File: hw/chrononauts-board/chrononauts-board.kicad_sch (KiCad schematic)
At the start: 56 parts, among them IC1 ESP32-C3-WROOM-02-N4, IC2 TLV62568DBVR, IC3 MXC6655XA, J1 73251-1290, J2 USB4105-GF-A, U1 CC1101RGP, Y1 NX3225GA-26MHZ

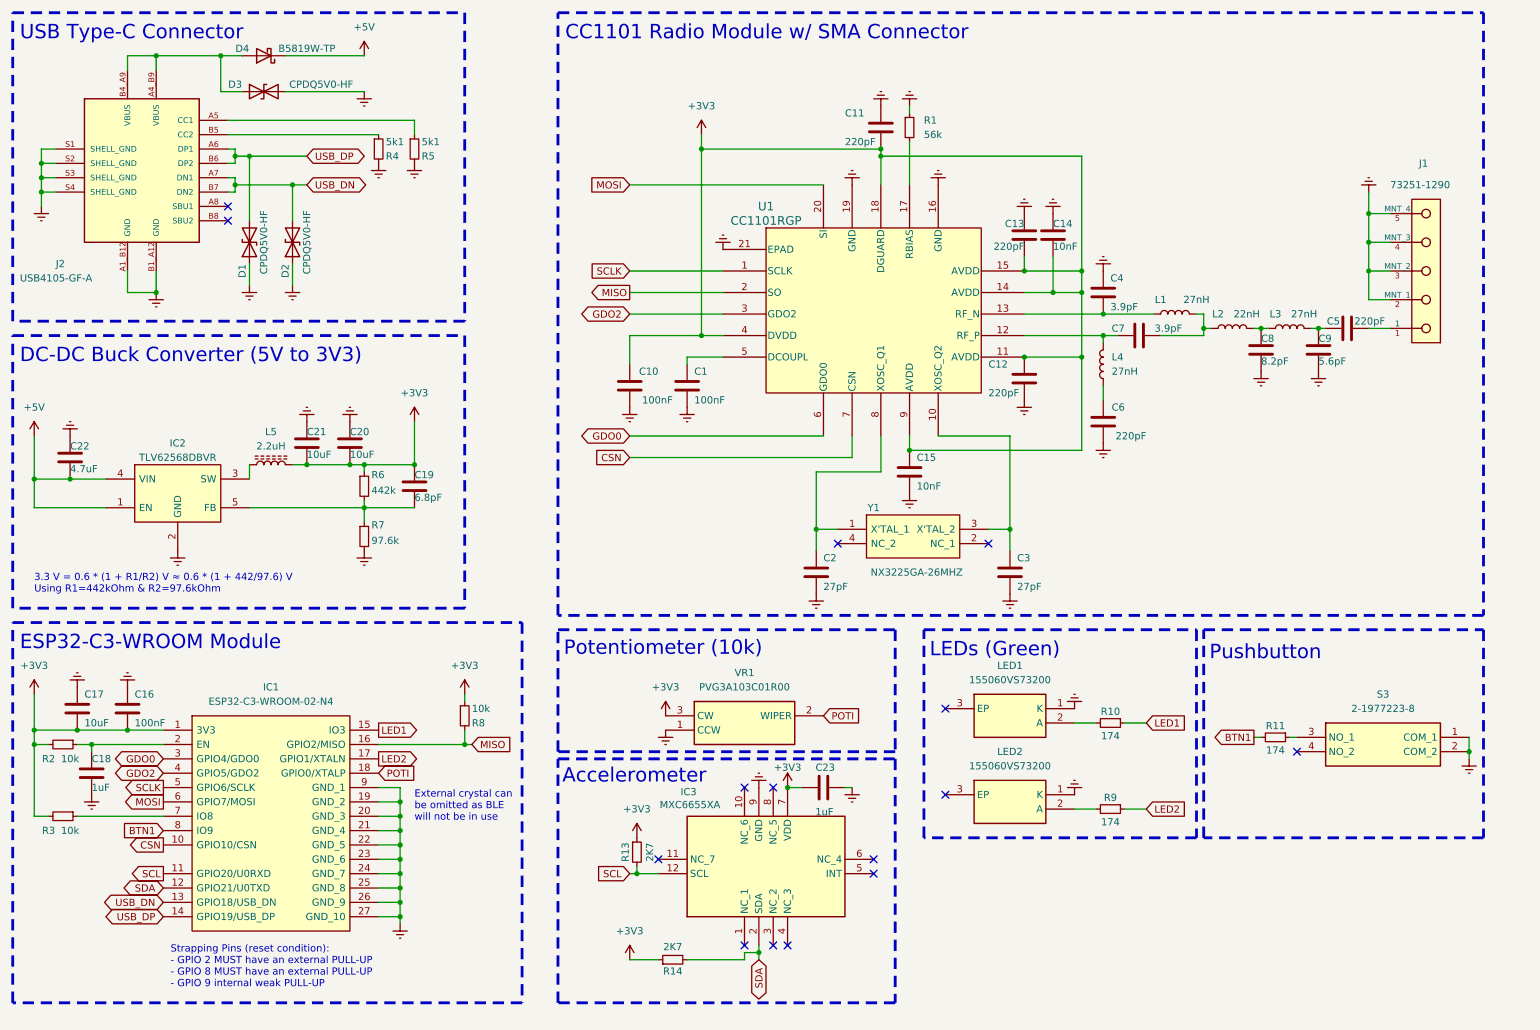
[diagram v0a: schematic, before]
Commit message: ready for production
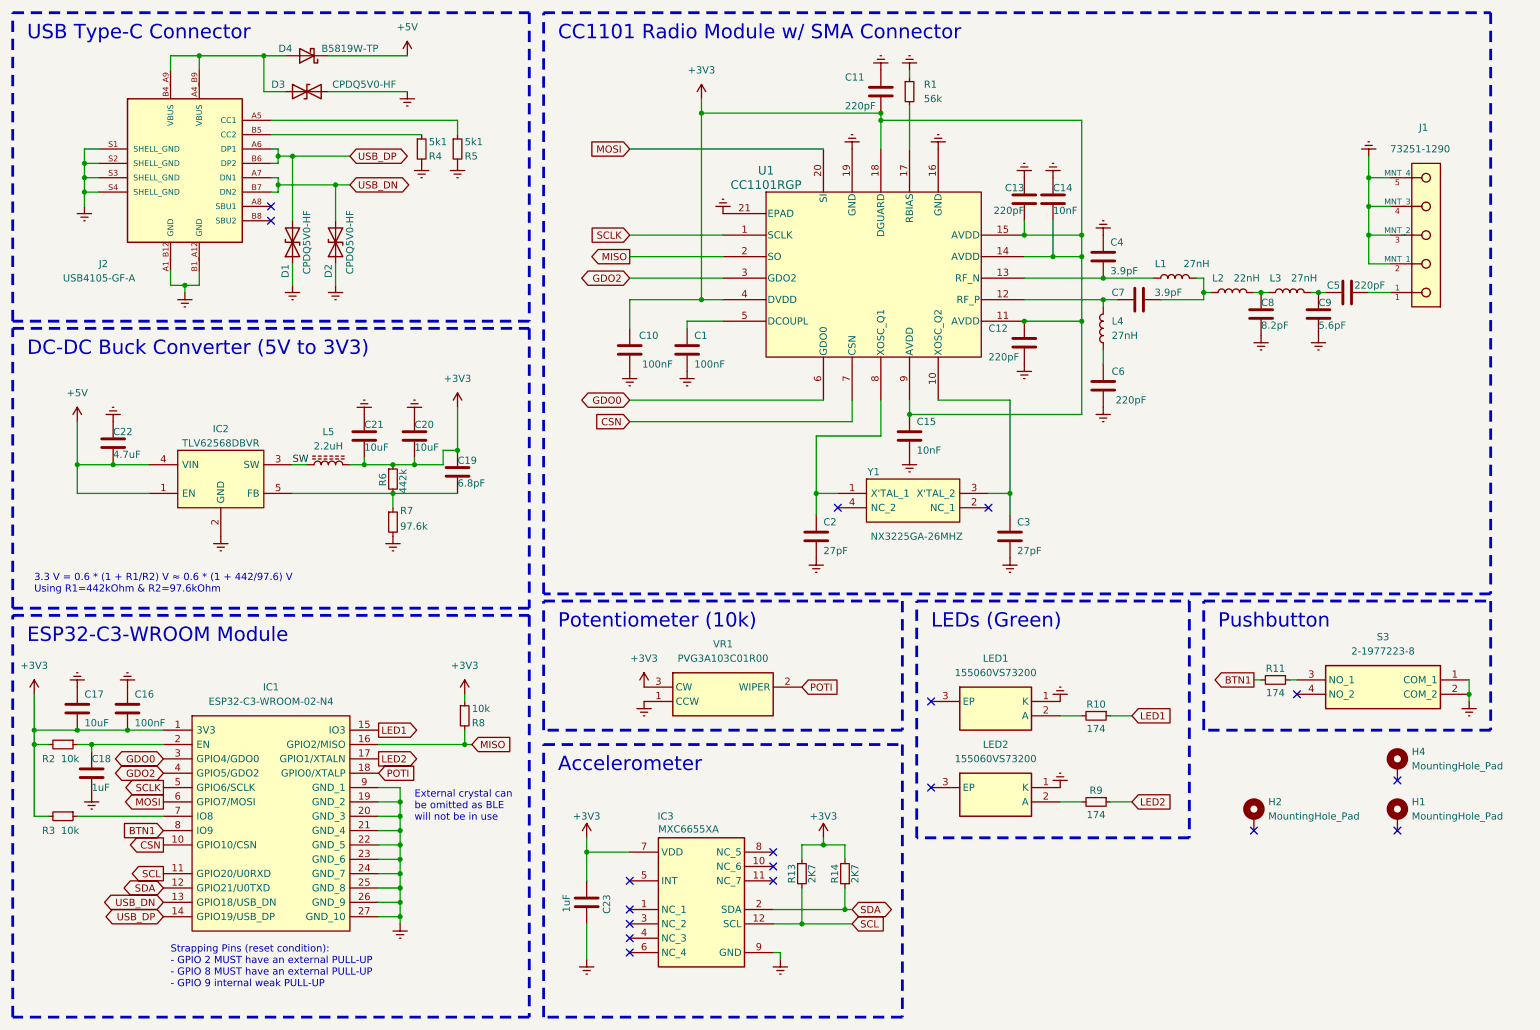
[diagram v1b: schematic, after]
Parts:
- added H1, H2, H4: MountingHole_Pad, MountingHole:MountingHole_2.2mm_M2_DIN965_Pad_TopBottom, symbol Mechanical:MountingHole_Pad
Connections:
- net +3V3: now also R14.2; no longer R14.1
- net SDA: now also R14.1; no longer R14.2
- net SW: now reaches IC2.3 (SW), L5.1
- no-connect marks 15 -> 18
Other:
- company: mineiwik -> chrononauts-quest
- moved on the sheet: C1, C10, C11, C12, C13, C14, C15, C19, C2, C20, C21, C22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

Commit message: generate production files
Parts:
- C1, C10, C16: LCSC (none) -> C431646
- C11, C12, C13, C5, C6: LCSC (none) -> C412611
- C14, C15: LCSC (none) -> C482489
- C17, C20, C21: LCSC (none) -> C510630
- C18, C23: LCSC (none) -> C527012
- C19: LCSC (none) -> C338054
- C2, C3: LCSC (none) -> C342944
- C22: LCSC (none) -> C77045
- C4, C7: LCSC (none) -> C565491
- C8: LCSC (none) -> C393674
- C9: LCSC (none) -> C525219
- D1, D2, D3: LCSC (none) -> C2441615
- D4: LCSC (none) -> C84354
- IC1: LCSC (none) -> C2934560
- IC2: LCSC (none) -> C163219
- IC3: LCSC (none) -> C5189050
- J2: LCSC (none) -> C3020560
- L1, L3, L4: LCSC (none) -> C12669
- L2: LCSC (none) -> C12670
- L5: LCSC (none) -> C2042636
- LED1, LED2: LCSC (none) -> C5362838
- R1: LCSC (none) -> C71703
- R10, R11, R9: LCSC (none) -> C416364
- R13, R14: LCSC (none) -> C416505
- R2, R3, R8: LCSC (none) -> C471764
- R4, R5: LCSC (none) -> C138073
- R6: LCSC (none) -> C234533
- R7: LCSC (none) -> C507495
- S3: LCSC (none) -> C2928194
- U1: LCSC (none) -> C29953
- VR1: LCSC (none) -> C840533
- Y1: LCSC (none) -> C485372
